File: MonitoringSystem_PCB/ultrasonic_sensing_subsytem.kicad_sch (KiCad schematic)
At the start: 36 parts, among them IC1 MAX660M_NOPB, J1 Ultrasonic_Conn_2, J3 Ultrasonic_Conn_1, U10 OPA192IDBVR, U11 TDC1000PW, U3 TDC7200PW, U5 OPA192IDBVR

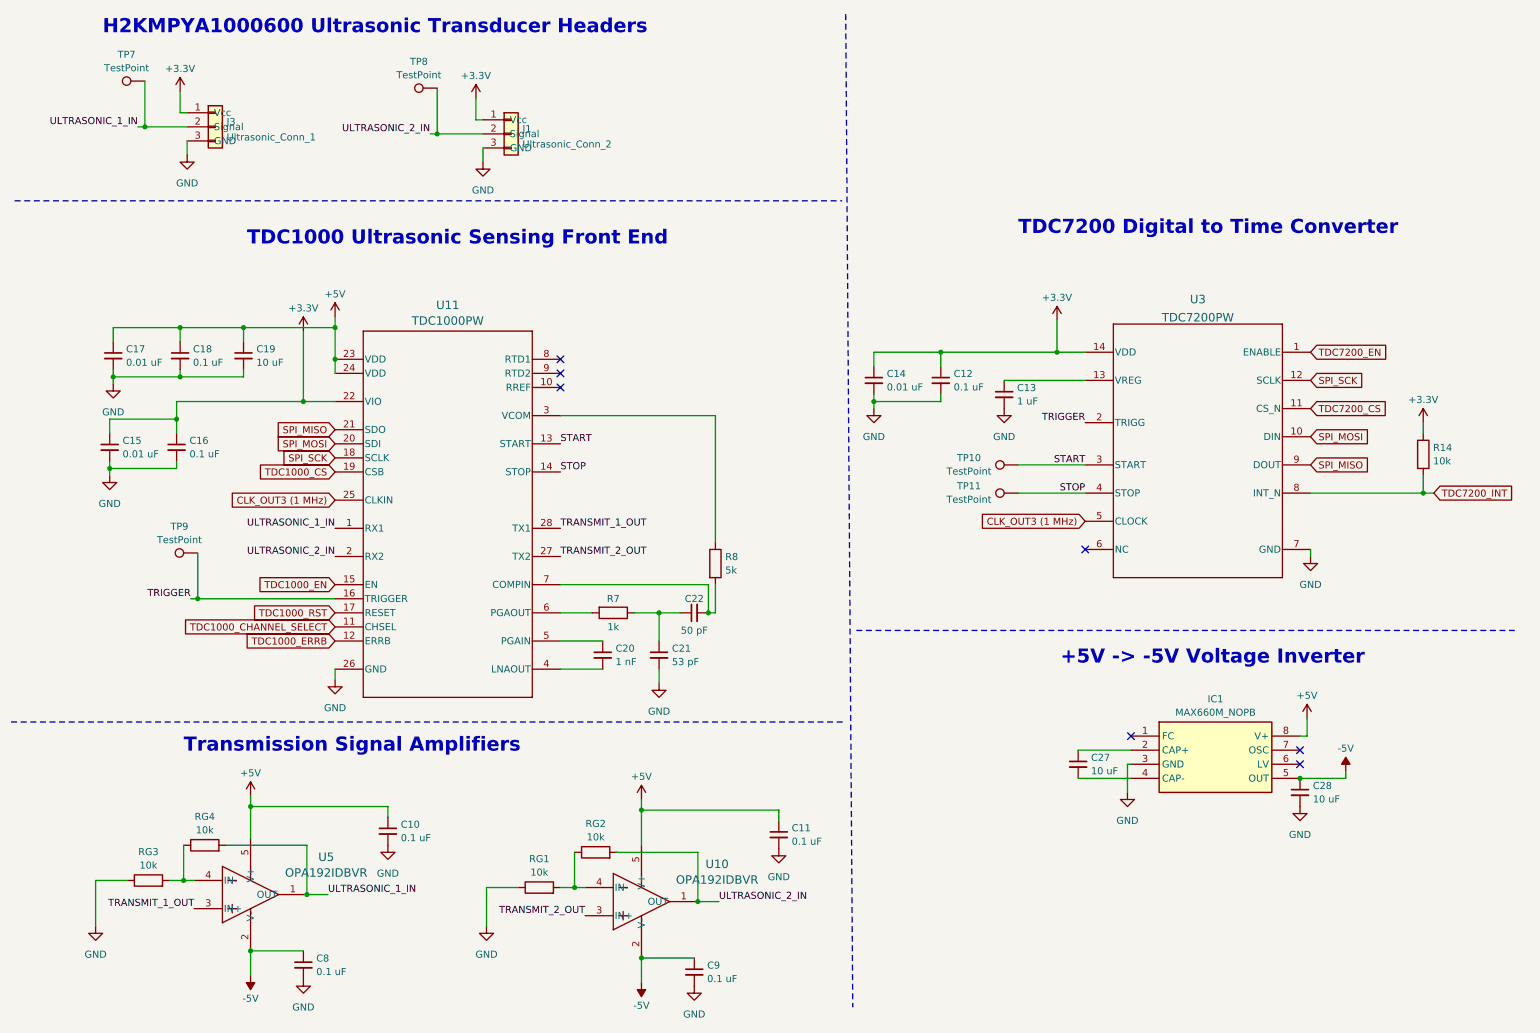
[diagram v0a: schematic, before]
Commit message: most recent pcb
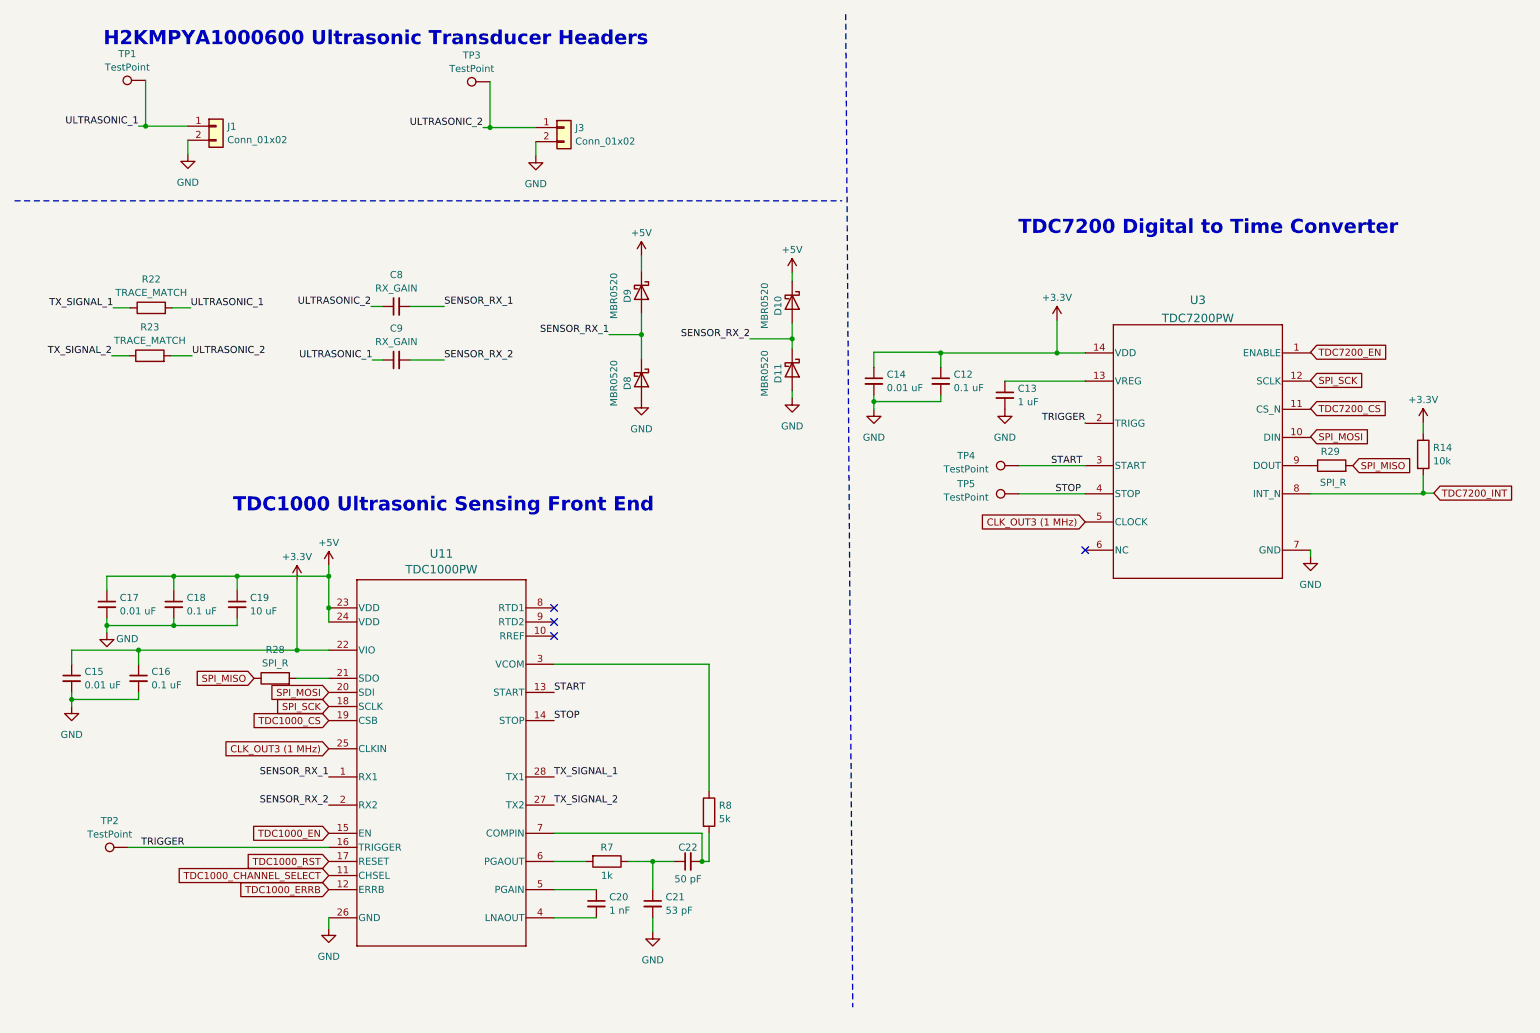
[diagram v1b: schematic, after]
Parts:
- removed C10, C11: 0.1 uF, Capacitor_SMD:C_0805_2012Metric, symbol Device:C_Small
- removed C27, C28: 10 uF, Capacitor_SMD:C_0805_2012Metric, symbol Device:C_Small
- removed IC1: MAX660M_NOPB, MAX660:SOIC127P600X175-8N, symbol Voltage Inverter:MAX660M_NOPB
- removed J1: Ultrasonic_Conn_2, Connector_Molex:Molex_KK-254_AE-6410-03A_1x03_P2.54mm_Vertical, symbol Connector_Generic:Conn_01x03
- removed J3: Ultrasonic_Conn_1, Connector_Molex:Molex_KK-254_AE-6410-03A_1x03_P2.54mm_Vertical, symbol Connector_Generic:Conn_01x03
- removed RG1, RG2, RG3, RG4: 10k, Resistor_SMD:R_0805_2012Metric, symbol Device:R
- removed TP10, TP11, TP7, TP8, TP9: TestPoint, TestPoint:TestPoint_Keystone_5010-5014_Multipurpose, symbol Connector:TestPoint
- removed U10, U5: OPA192IDBVR, OPA192IDBVR Amp:DBV0005A_N, symbol OPA192 AMP:OPA192IDBVR
- added D10, D11, D8, D9: MBR0520, Diode_SMD:D_SOD-123, symbol Diode:MBR0520
- added J1, J3: Conn_01x02, Connector_Molex:Molex_KK-254_AE-6410-02A_1x02_P2.54mm_Vertical, symbol Connector_Generic:Conn_01x02
- added R22, R23: TRACE_MATCH, Resistor_SMD:R_0805_2012Metric, symbol Device:R
- added R28, R29: SPI_R, Resistor_SMD:R_0805_2012Metric, symbol Device:R
- added TP1, TP2, TP3, TP4, TP5: TestPoint, TestPoint:TestPoint_Keystone_5010-5014_Multipurpose, symbol Connector:TestPoint
- C8, C9: value 0.1 uF -> RX_GAIN
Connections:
- net +5V: now also D10.1 (K), D9.1 (K)
- net GND: now also D11.2 (A), D8.2 (A), J1.2 (Pin_2), J3.2 (Pin_2); no longer C8.2, C9.2
- net SPI_MISO: now also R28.1, R29.2; no longer U11.21 (SDO), U3.9 (DOUT)
- net START: now also TP4.1
- net STOP: now also TP5.1
- net TRIGGER: now also TP2.1
- net -5V renamed ULTRASONIC_1
- net ULTRASONIC_1: now also J1.1 (Pin_1), R22.2, TP1.1; no longer C8.1
- net TRANSMIT_1_OUT renamed TX_SIGNAL_1
- net TX_SIGNAL_1: now also R22.1
- net TRANSMIT_2_OUT renamed TX_SIGNAL_2
- net TX_SIGNAL_2: now also R23.1
- net ULTRASONIC_1_IN renamed SENSOR_RX_1
- net SENSOR_RX_1: now also C8.2, D8.1 (K), D9.2 (A)
- net ULTRASONIC_2_IN renamed SENSOR_RX_2
- net SENSOR_RX_2: now also C9.2, D10.2 (A), D11.1 (K)
- new net: R29.1, U3.9 (DOUT)
- new net: R28.2, U11.21 (SDO)
- new net ULTRASONIC_2: C8.1, J3.1 (Pin_1), R23.2, TP3.1
- no-connect marks 7 -> 4
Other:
- note removed: "+5V -> -5V Voltage Inverter"
- note removed: "Transmission Signal Amplifiers"
- moved on the sheet: C15, C16, C17, C18, C19, C20, C21, C22, R7, R8, U11
